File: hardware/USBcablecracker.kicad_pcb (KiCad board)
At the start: 2 copper layers, 100 x 50 mm, 55 parts, among them P1 USB_A, P10 USB_A, P11 USB_B, P2 CONN_01X02, P3 USB_B-Micro, P7 USB_B-Mini, P8 USB_B-Micro-3.0, P9 USB_TYPEC-S, SW1 Switch_SPDT_x2, U1 ATmega32U4-AU, U2 LMV358, U3 AD623, Y1 16MHz

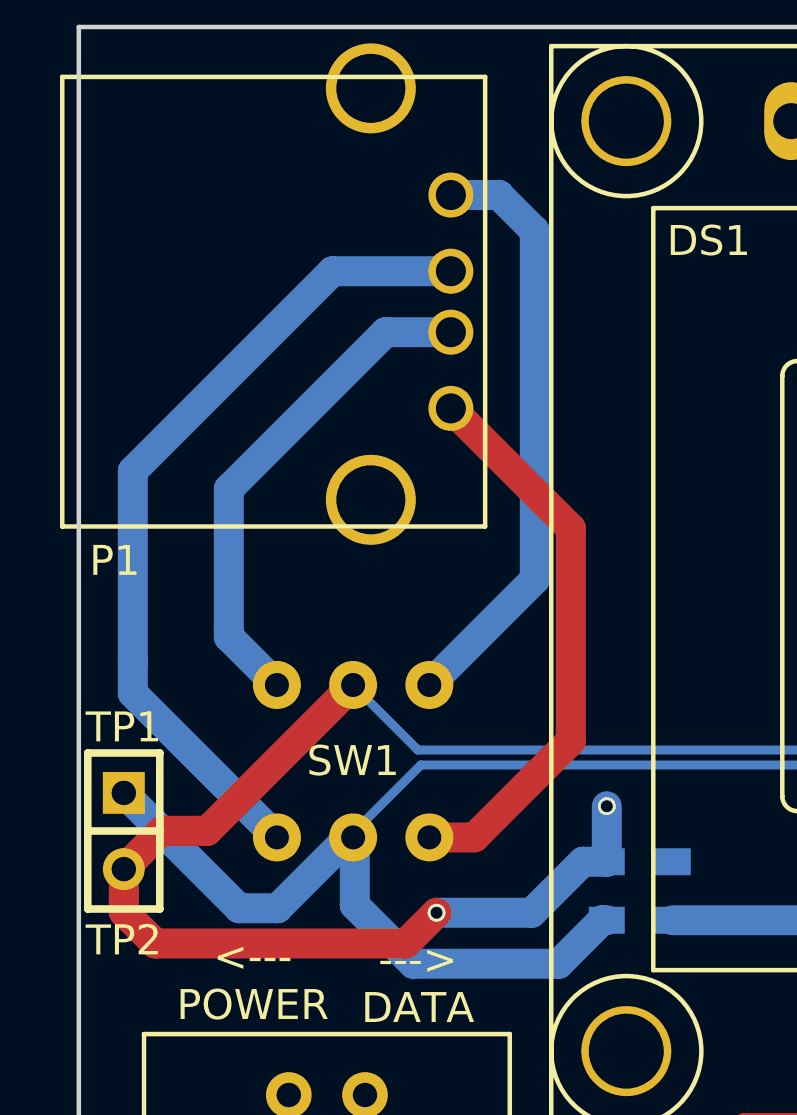
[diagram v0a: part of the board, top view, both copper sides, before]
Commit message: reverted to original switch
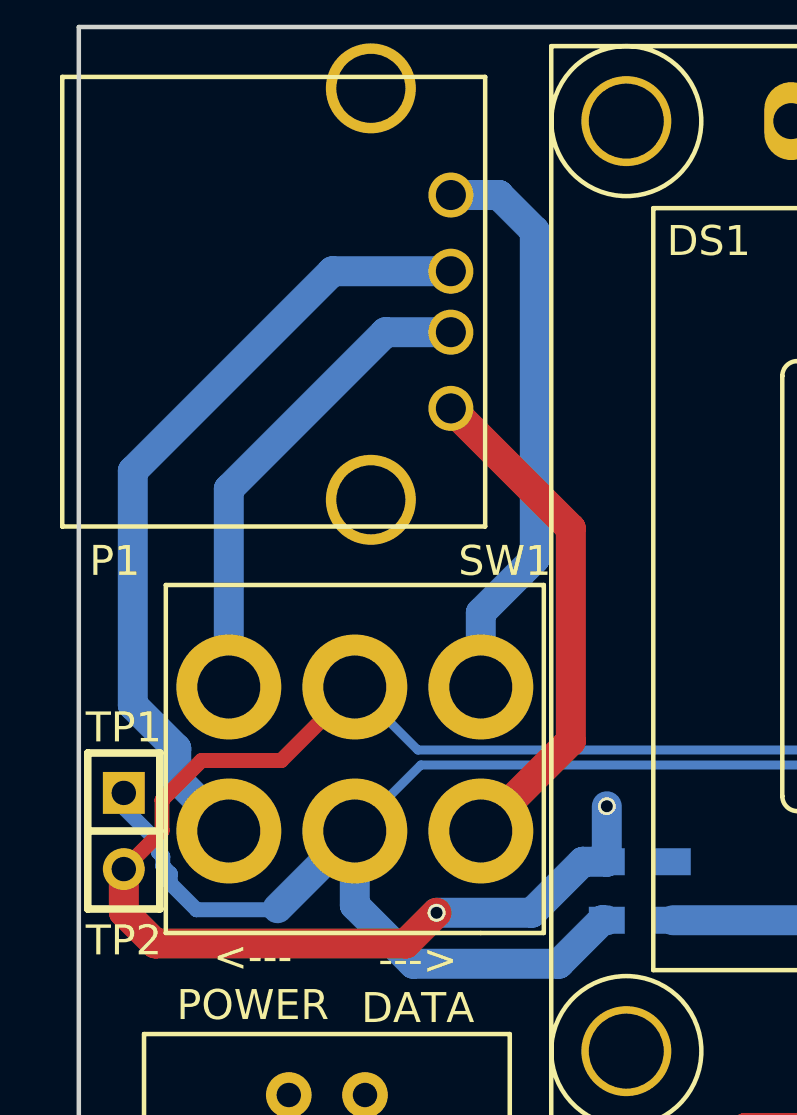
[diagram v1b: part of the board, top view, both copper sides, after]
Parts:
- SW1: footprint USBcablecracker:pin_headers_switch -> USBcablecracker:DPDT
- moved SW1 4.85 mm to (63.4, 76.8), turned to 90 degrees
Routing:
- net /TP2: track 93.2 -> 90.8 mm
- net Net-(P1-Pad4): track 18.8 -> 17.0 mm
- net /TP1: track 78.8 -> 79.8 mm
- net Net-(P1-Pad2): track 27.6 -> 26.7 mm
- net Net-(P1-Pad1): track 19.9 -> 19.2 mm
- net Net-(P1-Pad3): track 16.8 -> 16.2 mm
